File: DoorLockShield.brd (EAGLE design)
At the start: 68.6 x 63.4 mm, 21 parts, among them IC2 74HC595N, Q1 FDN5632N-F085, Q2 FDN5632N-F085

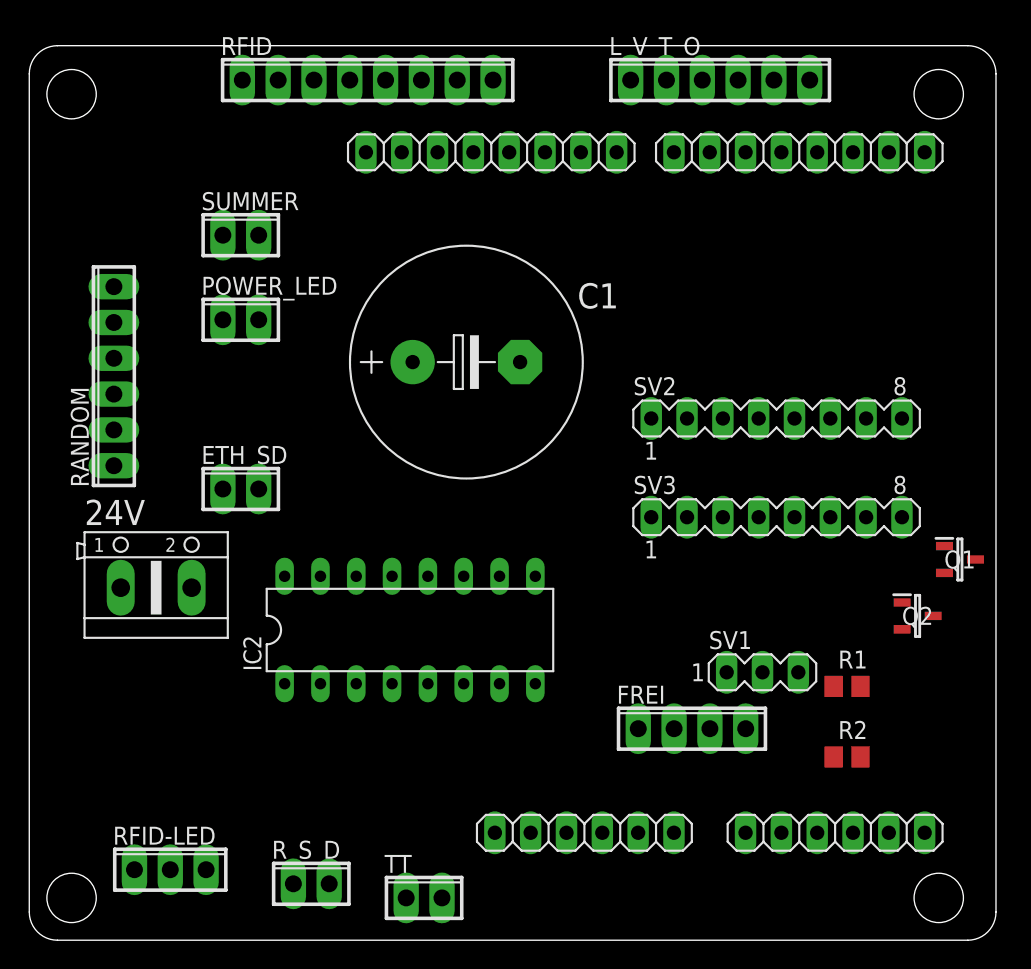
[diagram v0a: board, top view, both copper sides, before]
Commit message: started to add brd
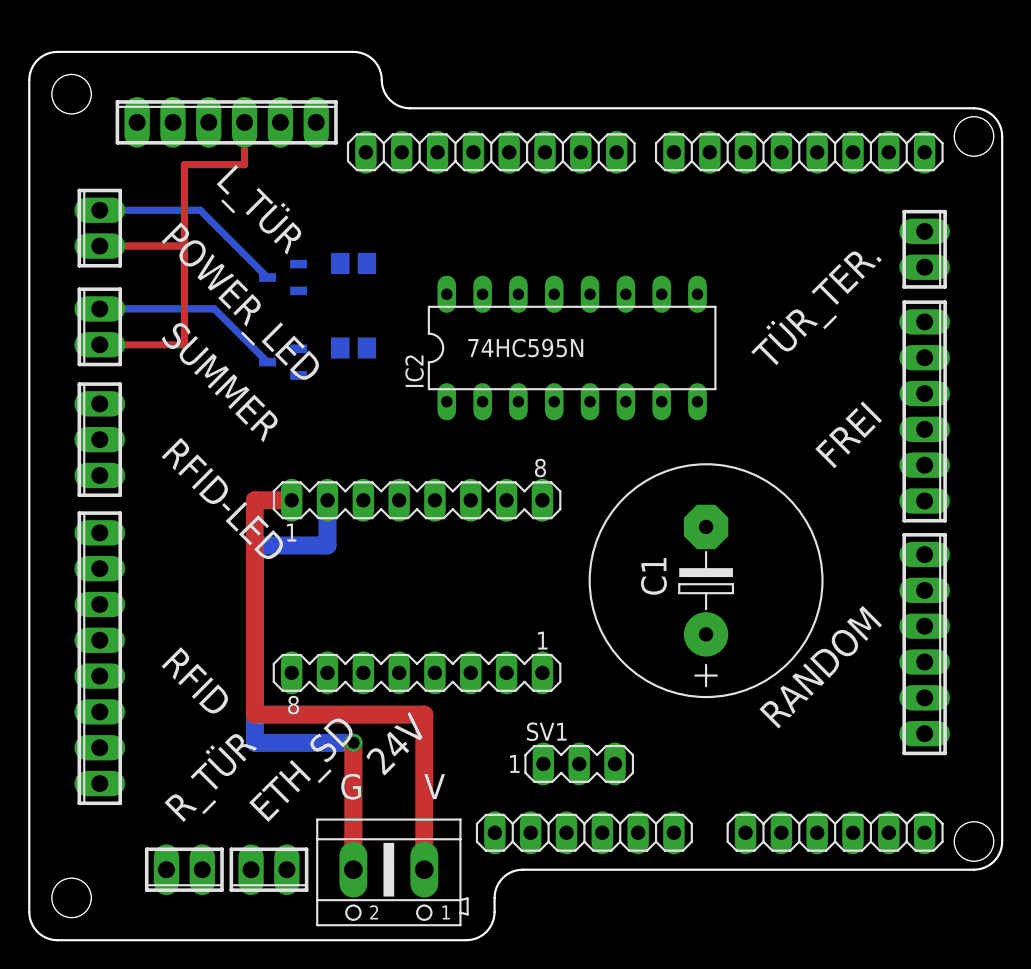
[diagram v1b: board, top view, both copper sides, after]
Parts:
- removed L_V_T_O: (no value), con-phoenix-254:6POL254
- removed R_S_D, TT: (no value), con-phoenix-254:2POL254
- added L_TÜR: (no value), con-phoenix-254:6POL254
- added R_TÜR, TÜR_TER.: (no value), con-phoenix-254:2POL254
- FREI: device con-phoenix-254:4POL254 -> con-phoenix-254:6POL254
- moved RANDOM 60.6 mm to (63.5, 21.0), turned to 270 degrees
- moved Q2 51.0 mm to (18.0, 47.0), flipped to the bottom
- moved Q1 50.0 mm to (18.0, 41.0), flipped to the bottom
- moved R2 49.5 mm to (23.0, 48.0), flipped to the bottom
- moved RFID 45.2 mm to (5.00, 20.0), turned to 90 degrees
- moved R1 42.4 mm to (23.0, 42.0), flipped to the bottom
- moved RFID-LED 30.9 mm to (5.00, 35.5), turned to 90 degrees
- moved FREI 27.9 mm to (63.5, 37.5), turned to 270 degrees
- moved SV3 27.8 mm to (27.5, 19.0), turned to 180 degrees
- moved ETH_SD 27.1 mm to (17.0, 5.00), turned to 180 degrees
- moved SV2 26.2 mm to (27.5, 31.2)
- moved 24V 25.9 mm to (25.5, 5.00), turned to 180 degrees
- moved IC2 23.1 mm to (38.5, 42.0)
- moved C1 23.0 mm to (48.0, 25.5), turned to 90 degrees
- moved SV1 14.5 mm to (39.0, 12.5)
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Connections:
- removed net GND: 24V.2, RANDOM.5, RANDOM.6
- new net GND24: 24V.2, SV2.2
- net 5V: now also FREI.5, L_TÜR.4, L_TÜR.5; no longer L_V_T_O.4, L_V_T_O.5
- net A0: now also L_TÜR.2; no longer L_V_T_O.2
- net A1: now also R_TÜR.2; no longer R_S_D.2
- net A2: now also L_TÜR.1; no longer L_V_T_O.1
- net A3: now also TÜR_TER..2; no longer TT.2
- net AGND: now also FREI.6, L_TÜR.6, RANDOM.5, RANDOM.6, R_TÜR.1, TÜR_TER..1; no longer L_V_T_O.6, R_S_D.1, SV2.2, TT.1
- net N$2: now also Q1.1; no longer Q2.1
- net N$3: now also Q2.1; no longer Q1.1
- net N$4: now also Q2.3; no longer Q1.3
- net N$5: now also Q1.3; no longer Q2.3
- net QD: now also L_TÜR.3; no longer L_V_T_O.3
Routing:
- net 24V: track 0.00 -> 40.8 mm
- net GND24: track 0.00 -> 38.4 mm, vias 0 -> 1
- net 5V: track 0.00 -> 32.0 mm
- net N$4: track 0.00 -> 13.9 mm
- net N$5: track 0.00 -> 13.5 mm
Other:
- board size 68.6 x 63.4 mm -> 69 x 63 mm
- board text added: "G"
- board text added: "V"
